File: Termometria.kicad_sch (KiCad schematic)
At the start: 60 parts, among them J1 Current_sense, U10 74HC74, U11 NE555D, U16 MPY634KU, U17 CD4052B, U18 ADA4898-2, U19 CD4052B, U7 ADA4898-2, U8 ADA4898-2, U9 ADA4898-2

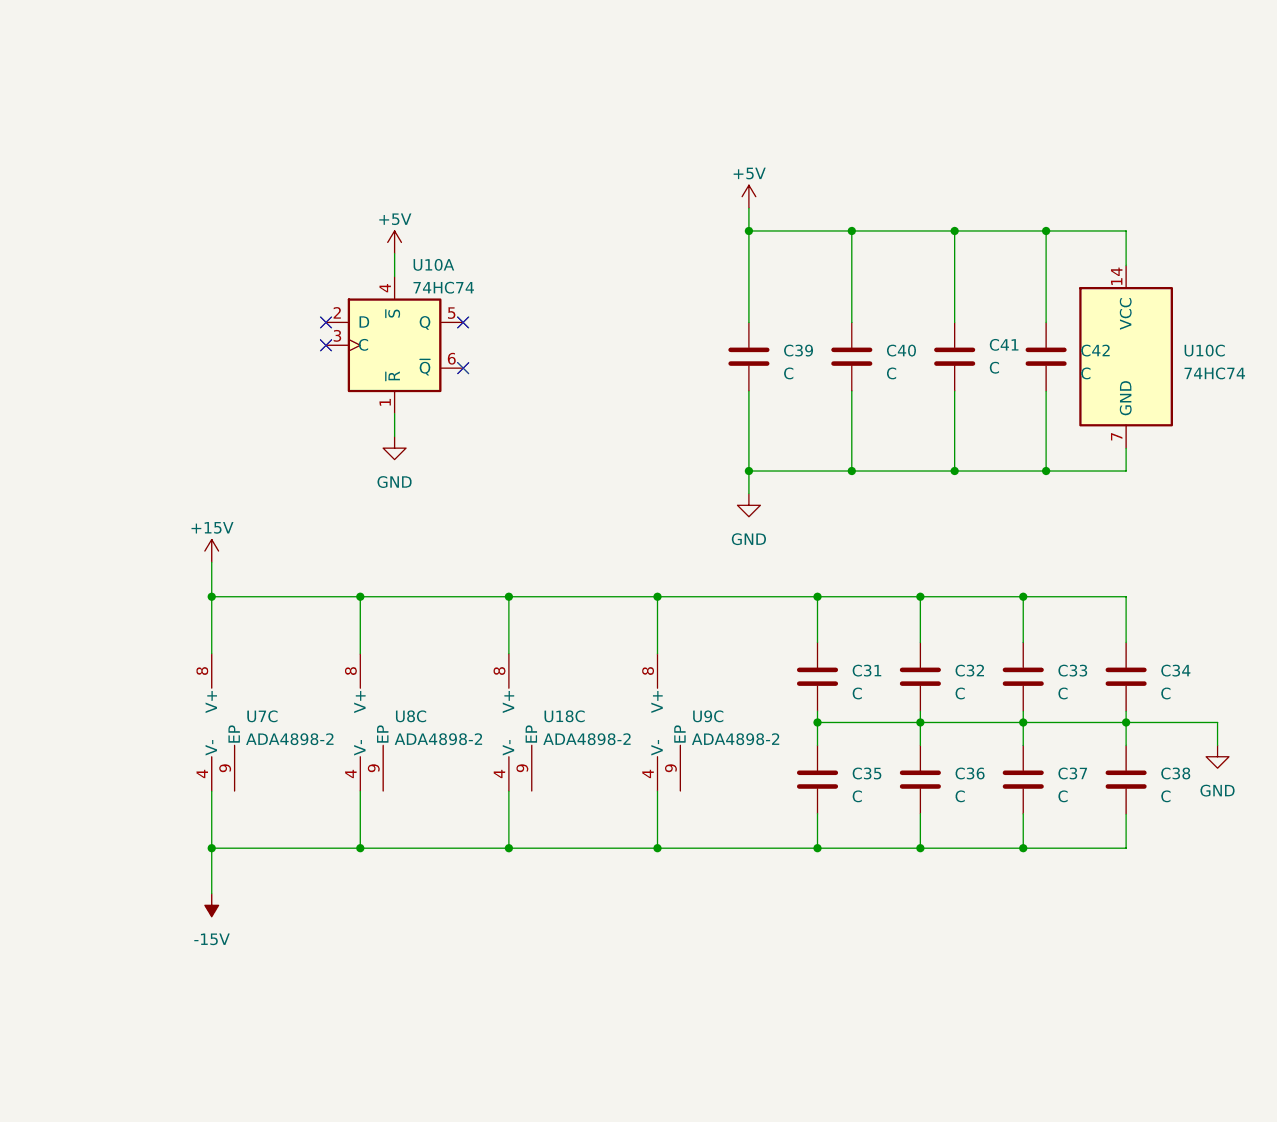
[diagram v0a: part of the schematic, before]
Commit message: first commit
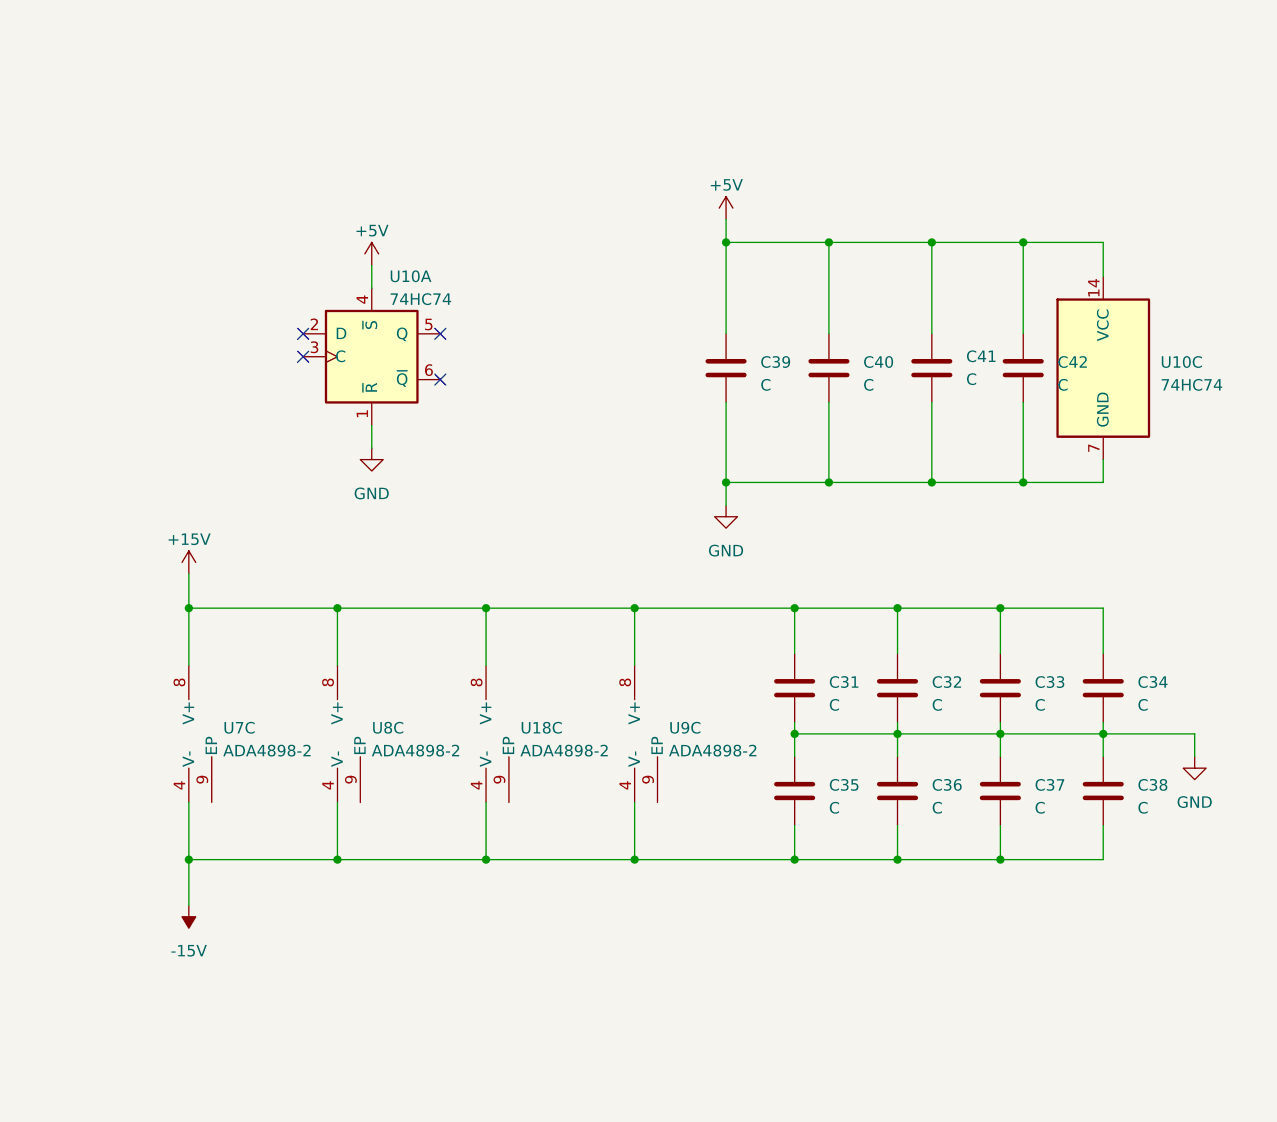
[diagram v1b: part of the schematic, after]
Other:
- moved on the sheet: C31, C32, C33, C34, C35, C36, C37, C38, C39, C40, C41, C42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
